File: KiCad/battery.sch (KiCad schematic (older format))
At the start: 7 parts, among them J1 Conn_01x07_Male, J2 Conn_01x01_Male, J3 Conn_01x01_Male, U1 ATtiny85-20SU, U2 LD1117S33TR_SOT223

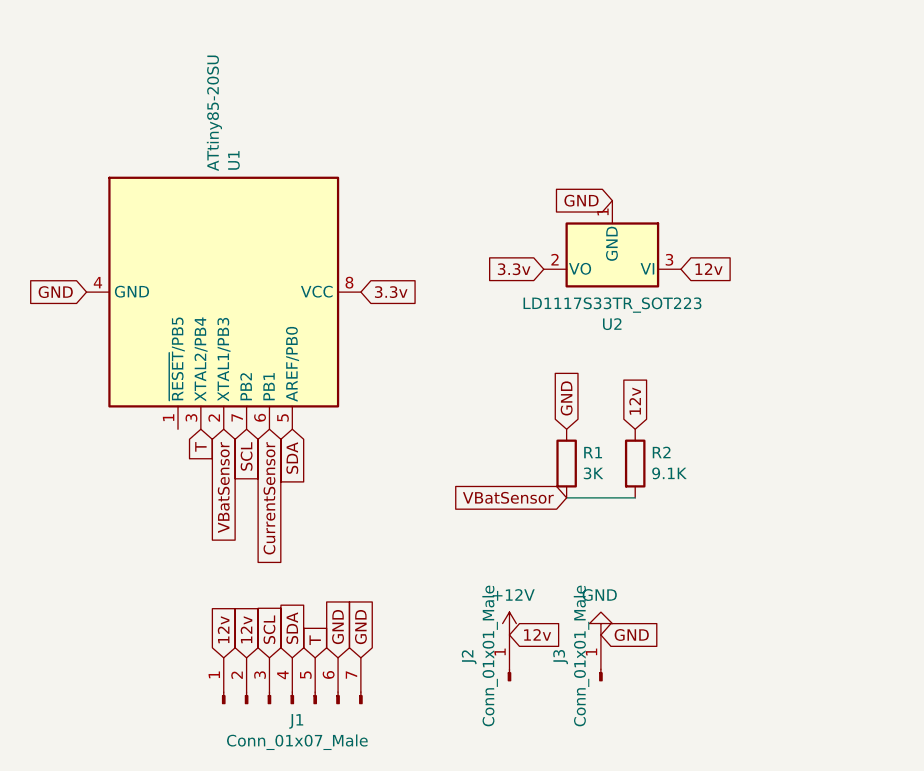
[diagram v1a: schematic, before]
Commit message: Update PCB before manufacturing
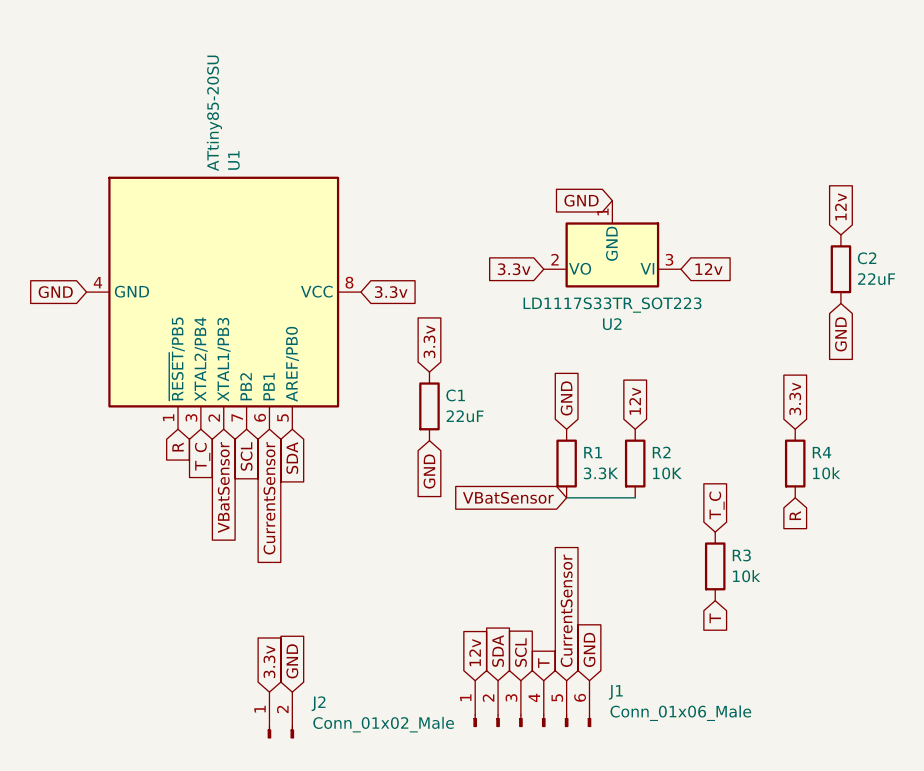
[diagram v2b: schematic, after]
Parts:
- removed J1: Conn_01x07_Male, Connector_PinHeader_2.54mm:PinHeader_1x07_P2.54mm_Vertical, symbol Connector:Conn_01x07_Male
- removed J2, J3: Conn_01x01_Male, Connector_Pin:Pin_D1.4mm_L8.5mm_W2.8mm_FlatFork, symbol Connector:Conn_01x01_Male
- added C1, C2: 22uF, Capacitor_SMD:C_0805_2012Metric, symbol Device:R
- added J1: Conn_01x06_Male, Connector_PinHeader_2.54mm:PinHeader_1x06_P2.54mm_Horizontal, symbol Connector:Conn_01x06_Male
- added J2: Conn_01x02_Male, Connector_PinHeader_2.54mm:PinHeader_1x02_P2.54mm_Vertical, symbol Connector:Conn_01x02_Male
- added R3, R4: 10k, Resistor_SMD:R_0402_1005Metric, symbol Device:R
- R1: value 3K -> 3.3K; footprint Parts:R_1206_3216Metric_Pad1.42x1.75mm_HandSolder -> Resistor_SMD:R_0402_1005Metric
- R2: value 9.1K -> 10K; footprint Parts:R_1206_3216Metric_Pad1.42x1.75mm_HandSolder -> Resistor_SMD:R_0402_1005Metric
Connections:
- net 3.3v: now also C1.1, J2.1 (Pin_1), R4.1
- net CurrentSensor: now also J1.5 (Pin_5)
- net GND: now also C1.2, C2.2, J1.6 (Pin_6), J2.2 (Pin_2)
- net SCL: now also J1.3 (Pin_3)
- net SDA: now also J1.2 (Pin_2)
- net T: now also J1.4 (Pin_4), R3.2; no longer U1.3 (XTAL2/PB4)
- net R: now reaches U1.1 (~RESET~/PB5)
- net R: now also R4.2
- net +12V renamed 12v
- net 12v: now also C2.1, J1.1 (Pin_1)
- new net T_C: R3.1, U1.3 (XTAL2/PB4)
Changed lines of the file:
@@
 EESchema Schematic File Version 4
-LIBS:battery-cache
-EELAYER 26 0
+EELAYER 30 0
 EELAYER END
 $Descr A4 11693 8268
@@
 P 4600 2500
 F 0 "R2" H 4670 2546 50  0000 L CNN
-F 1 "9.1K" H 4670 2455 50  0000 L CNN
-F 2 "Parts:R_1206_3216Metric_Pad1.42x1.75mm_HandSolder" V 4530 2500 50  0001 C CNN
+F 1 "10K" H 4670 2455 50  0000 L CNN
+F 2 "Resistor_SMD:R_0402_1005Metric" V 4530 2500 50  0001 C CNN
 F 3 "~" H 4600 2500 50  0001 C CNN
 	1    4600 2500
@@
 P 4300 2500
 F 0 "R1" H 4370 2546 50  0000 L CNN
-F 1 "3K" H 4370 2455 50  0000 L CNN
-F 2 "Parts:R_1206_3216Metric_Pad1.42x1.75mm_HandSolder" V 4230 2500 50  0001 C CNN
+F 1 "3.3K" H 4370 2455 50  0000 L CNN
+F 2 "Resistor_SMD:R_0402_1005Metric" V 4230 2500 50  0001 C CNN
 F 3 "~" H 4300 2500 50  0001 C CNN
 	1    4300 2500
 	1    0    0    -1
 $EndComp
-$Comp
-L power:GND #PWR0101
-U 1 1 5EC353CA
-P 4450 3250
-F 0 "#PWR0101" H 4450 3000 50  0001 C CNN
-F 1 "GND" H 4455 3077 50  0000 C CNN
-F 2 "" H 4450 3250 50  0001 C CNN
-F 3 "" H 4450 3250 50  0001 C CNN
-	1    4450 3250
-	-1   0    0    1
-$EndComp
-$Comp
-L Connector:Conn_01x07_Male J1
-U 1 1 5EC62E55
-P 3100 3550
-F 0 "J1" V 3027 3528 50  0000 C CNN
-F 1 "Conn_01x07_Male" V 2936 3528 50  0000 C CNN
-F 2 "Connector_PinHeader_2.54mm:PinHeader_1x07_P2.54mm_Vertical" H 3100 3550 50  0001 C CNN
-F 3 "~" H 3100 3550 50  0001 C CNN
-	1    3100 3550
-	0    -1   -1   0
-$EndComp
-Text GLabel 2800 3350 1    50   Input ~ 0
+Text GLabel 3900 3450 1    50   Input ~ 0
 12v
-Text GLabel 2900 3350 1    50   Input ~ 0
-12v
-Text GLabel 3000 3350 1    50   Input ~ 0
-SCL
-Text GLabel 3100 3350 1    50   Input ~ 0
-SDA
-Text GLabel 3200 3350 1    50   Input ~ 0
-T
-Text GLabel 3300 3350 1    50   Input ~ 0
-GND
-Text GLabel 3400 3350 1    50   Input ~ 0
+Text GLabel 4400 3450 1    50   Input ~ 0
 GND
 $Comp
@@
 	-1   0    0    1
 $EndComp
-$Comp
-L power:+12V #PWR0102
-U 1 1 5EC34276
-P 4050 3250
-F 0 "#PWR0102" H 4050 3100 50  0001 C CNN
-F 1 "+12V" H 4065 3423 50  0000 C CNN
-F 2 "" H 4050 3250 50  0001 C CNN
-F 3 "" H 4050 3250 50  0001 C CNN
-	1    4050 3250
-	1    0    0    -1
-$EndComp
-Text GLabel 4050 3250 2    50   Input ~ 0
-12v
-Text GLabel 4450 3250 2    50   Input ~ 0
-GND
 Text GLabel 4800 1650 2    50   Input ~ 0
 12v
@@
 $EndComp
 Text GLabel 2700 2350 3    50   Input ~ 0
-T
+T_C
 Text GLabel 2900 2350 3    50   Input ~ 0
 SCL
@@
 SDA
 $Comp
-L Connector:Conn_01x01_Male J2
-U 1 1 5ECDB575
-P 4050 3450
-F 0 "J2" H 4158 3631 50  0000 C CNN
-F 1 "Conn_01x01_Male" H 4158 3540 50  0000 C CNN
-F 2 "Connector_Pin:Pin_D1.4mm_L8.5mm_W2.8mm_FlatFork" H 4050 3450 50  0001 C CNN
-F 3 "~" H 4050 3450 50  0001 C CNN
-	1    4050 3450
+L Device:R R4
+U 1 1 5F803F9D
+P 5300 2500
+F 0 "R4" H 5370 2546 50  0000 L CNN
+F 1 "10k" H 5370 2455 50  0000 L CNN
+F 2 "Resistor_SMD:R_0402_1005Metric" V 5230 2500 50  0001 C CNN
+F 3 "~" H 5300 2500 50  0001 C CNN
+	1    5300 2500
+	1    0    0    -1
+$EndComp
+Text GLabel 2600 2350 3    50   Input ~ 0
+R
+Text GLabel 5300 2650 3    50   Input ~ 0
+R
+Text GLabel 5300 2350 1    50   Input ~ 0
+3.3v
+$Comp
+L Device:R C1
+U 1 1 5F8051D0
+P 3700 2250
+F 0 "C1" H 3770 2296 50  0000 L CNN
+F 1 "22uF" H 3770 2205 50  0000 L CNN
+F 2 "Capacitor_SMD:C_0805_2012Metric" V 3630 2250 50  0001 C CNN
+F 3 "~" H 3700 2250 50  0001 C CNN
+	1    3700 2250
+	1    0    0    -1
+$EndComp
+Text GLabel 3700 2100 1    50   Input ~ 0
+3.3v
+Text GLabel 3700 2400 3    50   Input ~ 0
+GND
+Text GLabel 4200 3450 1    50   Input ~ 0
+T
+$Comp
+L Device:R R3
+U 1 1 5F813E79
+P 4950 2950
+F 0 "R3" H 5020 2996 50  0000 L CNN
+F 1 "10k" H 5020 2905 50  0000 L CNN
+F 2 "Resistor_SMD:R_0402_1005Metric" V 4880 2950 50  0001 C CNN
+F 3 "~" H 4950 2950 50  0001 C CNN
+	1    4950 2950
+	1    0    0    -1
+$EndComp
+Text GLabel 4950 3100 3    50   Input ~ 0
+T
+Text GLabel 4950 2800 1    50   Input ~ 0
+T_C
+$Comp
+L Connector:Conn_01x06_Male J1
+U 1 1 5F8168A9
+P 4100 3650
+F 0 "J1" V 4254 3262 50  0000 R CNN
+F 1 "Conn_01x06_Male" V 4163 3262 50  0000 R CNN
+F 2 "Connector_PinHeader_2.54mm:PinHeader_1x06_P2.54mm_Horizontal" H 4100 3650 50  0001 C CNN
+F 3 "~" H 4100 3650 50  0001 C CNN
+	1    4100 3650
 	0    -1   -1   0
 $EndComp
+Text GLabel 4300 3450 1    50   Input ~ 0
+CurrentSensor
+Text GLabel 4100 3450 1    50   Input ~ 0
+SCL
+Text GLabel 4000 3450 1    50   Input ~ 0
+SDA
 $Comp
-L Connector:Conn_01x01_Male J3
-U 1 1 5ECDC6DD
-P 4450 3450
-F 0 "J3" H 4558 3631 50  0000 C CNN
-F 1 "Conn_01x01_Male" H 4558 3540 50  0000 C CNN
-F 2 "Connector_Pin:Pin_D1.4mm_L8.5mm_W2.8mm_FlatFork" H 4450 3450 50  0001 C CNN
-F 3 "~" H 4450 3450 50  0001 C CNN
-	1    4450 3450
+L Device:R C2
+U 1 1 5F823DED
+P 5500 1650
+F 0 "C2" H 5570 1696 50  0000 L CNN
+F 1 "22uF" H 5570 1605 50  0000 L CNN
+F 2 "Capacitor_SMD:C_0805_2012Metric" V 5430 1650 50  0001 C CNN
+F 3 "~" H 5500 1650 50  0001 C CNN
+	1    5500 1650
+	1    0    0    -1
+$EndComp
+Text GLabel 5500 1500 1    50   Input ~ 0
+12v
+Text GLabel 5500 1800 3    50   Input ~ 0
+GND
+$Comp
+L Connector:Conn_01x02_Male J2
+U 1 1 5F81605B
+P 3000 3700
+F 0 "J2" V 3154 3512 50  0000 R CNN
+F 1 "Conn_01x02_Male" V 3063 3512 50  0000 R CNN
+F 2 "Connector_PinHeader_2.54mm:PinHeader_1x02_P2.54mm_Vertical" H 3000 3700 50  0001 C CNN
+F 3 "~" H 3000 3700 50  0001 C CNN
+	1    3000 3700
 	0    -1   -1   0
 $EndComp
+Text GLabel 3000 3500 1    50   Input ~ 0
+3.3v
+Text GLabel 3100 3500 1    50   Input ~ 0
+GND
 $EndSCHEMATC
